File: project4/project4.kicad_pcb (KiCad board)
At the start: 2 copper layers, 33 parts, among them J1 Conn_02x03_Odd_Even, J2 Conn_02x03_Odd_Even, J3 Conn_02x03_Odd_Even, J4 Conn_02x03_Odd_Even, J5 Conn_02x03_Odd_Even, J6 Conn_02x02_Odd_Even, U1 SST27ST020, U2 SST27ST020, U3 SST27ST020, U4 SST27ST020, U5 74LS139, U6 74LS32, U7 74LS00, U8 74LS670, U9 74LS670

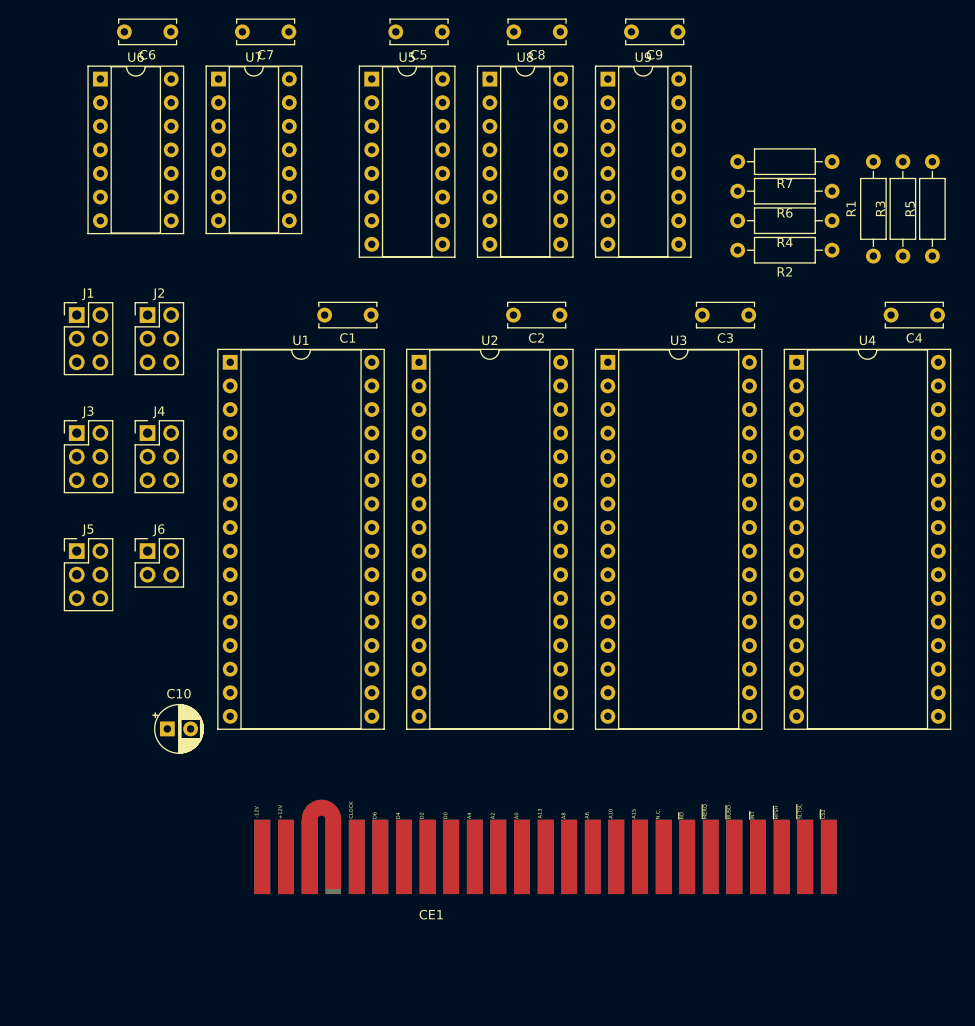
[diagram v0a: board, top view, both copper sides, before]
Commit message: Modified PCB 4
Signed-off-by: ykp74 <ykp7409@gmail.com>
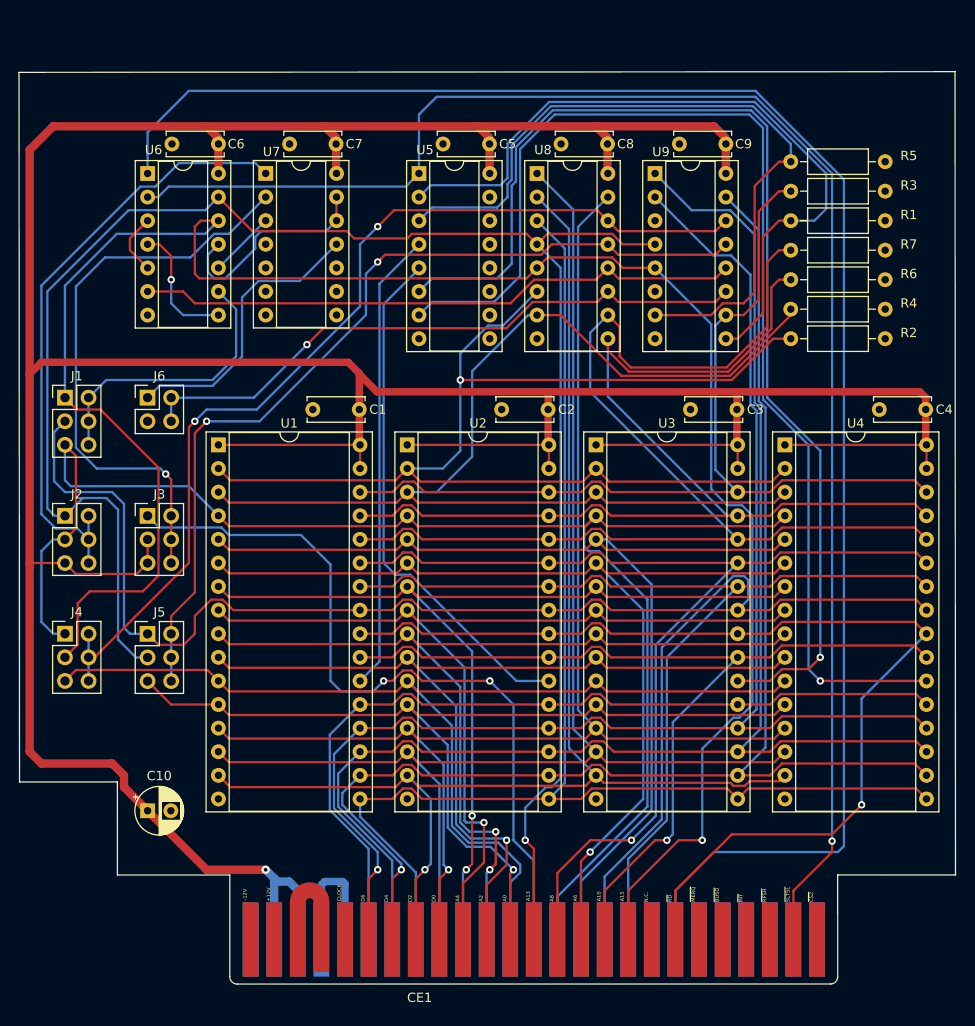
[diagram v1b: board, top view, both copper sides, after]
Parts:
- J1, J2, J3, J4, J5: value Conn_02x03_Odd_Even -> Conn_02x03
- J6: value Conn_02x02_Odd_Even -> Conn_02x02
- moved J2 23.4 mm to (94.0, 100.3)
- moved J4 23.4 mm to (94.0, 113.0)
- moved J6 16.5 mm to (102.9, 87.6)
- moved C9 13.1 mm to (165.1, 60.3)
- moved C6 13.1 mm to (110.5, 60.3)
- moved C7 13.1 mm to (123.2, 60.3)
- moved C8 13.1 mm to (152.4, 60.3)
- moved C5 13.1 mm to (139.7, 60.3)
- moved J3 11.7 mm to (102.9, 100.3)
- moved J5 11.7 mm to (102.9, 113.0)
- moved U8 11.4 mm to (144.8, 63.5)
- moved R5 11.4 mm to (182.2, 62.2), turned to 180 degrees
- moved U5 11.4 mm to (132.1, 63.5)
- moved U6 11.4 mm to (102.9, 63.5)
- moved U7 11.4 mm to (115.6, 63.5)
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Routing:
- net +5V: track 0.00 -> 422.0 mm, vias 0 -> 1
- net /A15: track 0.00 -> 216.5 mm, vias 0 -> 1
- net /A13: track 0.00 -> 201.8 mm, vias 0 -> 1
- net //WR: track 0.00 -> 182.3 mm
- net /A11: track 0.00 -> 172.7 mm
- net //SLTSL: track 0.00 -> 169.4 mm, vias 0 -> 1
- net /A12: track 0.00 -> 164.2 mm
- net /D5: track 0.00 -> 157.7 mm
- net /D6: track 0.00 -> 153.8 mm, vias 0 -> 1
- net /D4: track 0.00 -> 150.6 mm, vias 0 -> 1
- net /D1: track 0.00 -> 150.3 mm
- net /D2: track 0.00 -> 148.1 mm, vias 0 -> 1
- net /D0: track 0.00 -> 148.0 mm, vias 0 -> 1
- net /D3: track 0.00 -> 145.6 mm
- net /MA16: track 0.00 -> 129.8 mm, vias 0 -> 1
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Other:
- board outline added: 100.8 x 98.2 mm
